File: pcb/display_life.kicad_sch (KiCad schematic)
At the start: 50 parts, among them J3 1st Bit_shifter, J4 1st 7 Segment, J5 2nd Bit_shifter, J6 2nd 7 Segment, J7 decoder_input, J8 disp_1_decoder, J9 disp_2_decoder, Q1 Q_NPN_CBE, Q2 Q_NPN_CBE, Q3 Q_NPN_CBE, Q4 Q_NPN_CBE, Q5 Q_NPN_CBE, Q6 Q_NPN_CBE, Q7 Q_NPN_CBE, Q8 Q_NPN_CBE, U2 74HC595, U3 74HC595, U4 4028, U5 CC56-12SURKWA, U6 CC56-12SURKWA

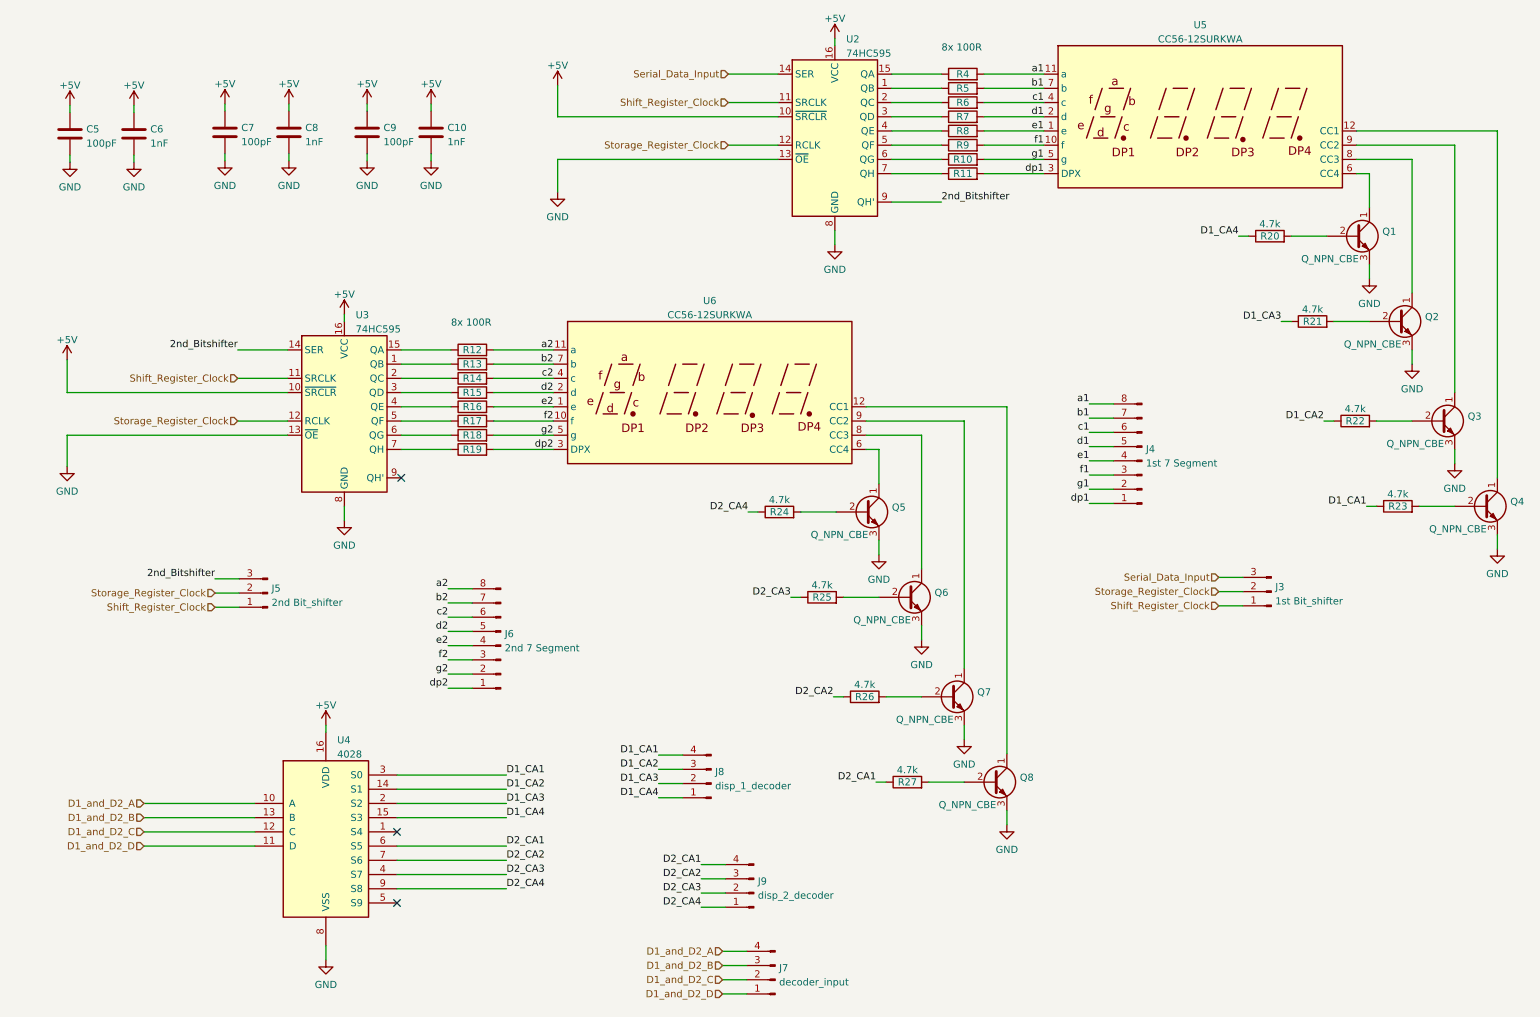
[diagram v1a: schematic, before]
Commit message: new parts and stuff
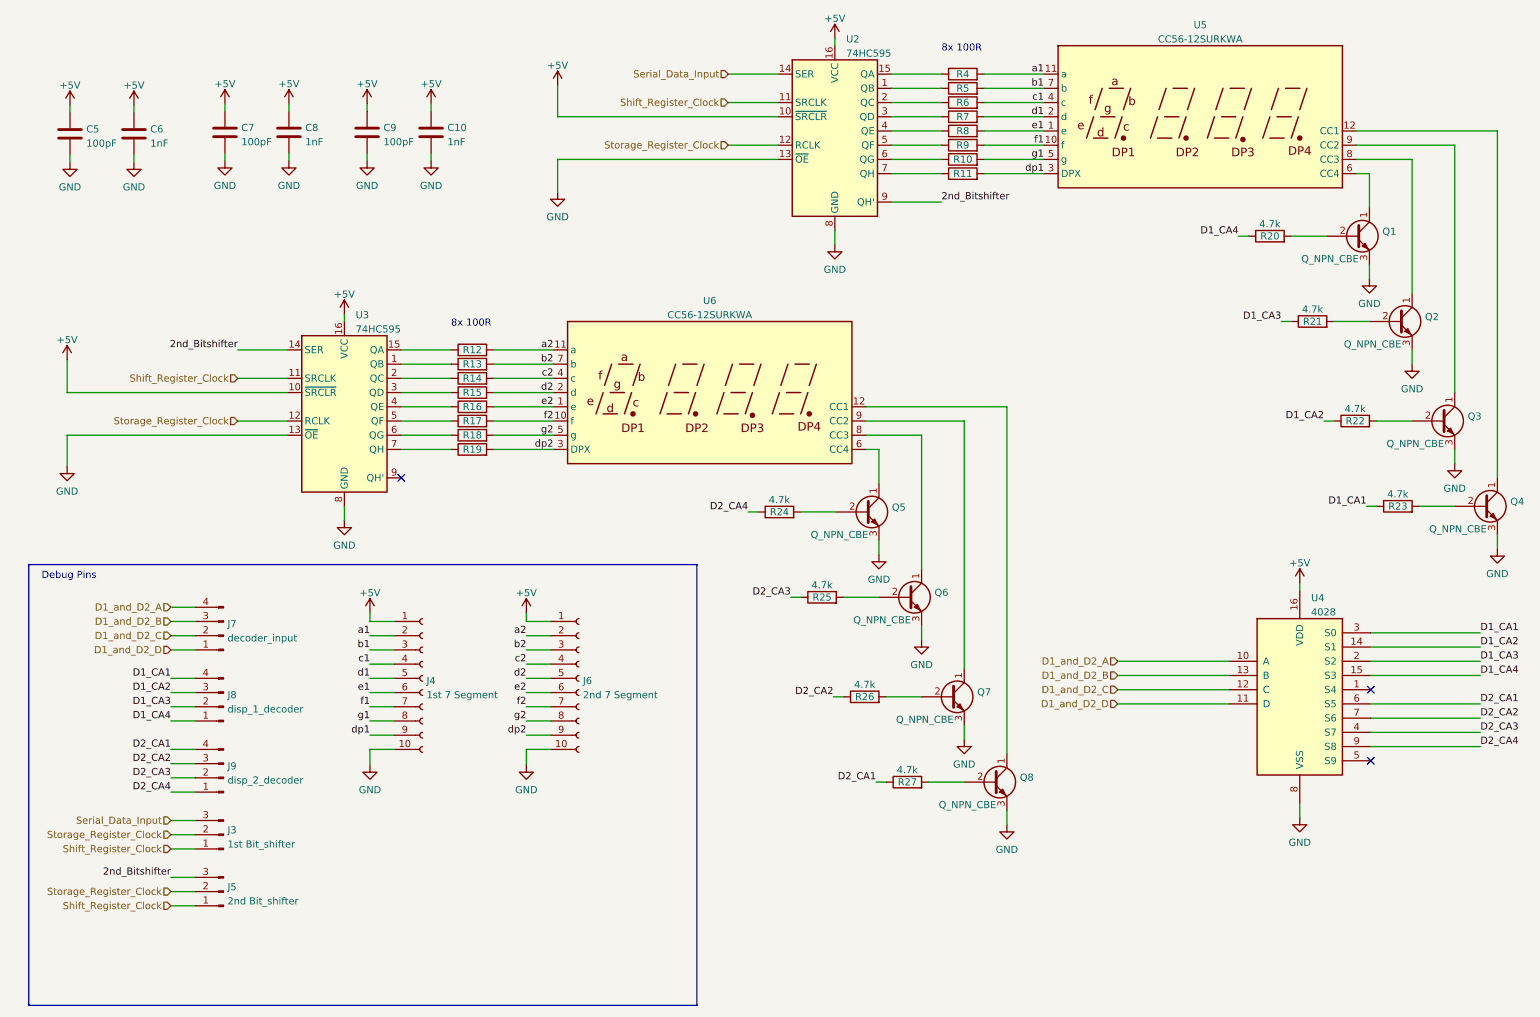
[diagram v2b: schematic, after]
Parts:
- removed J4: 1st 7 Segment, Connector_PinHeader_2.54mm:PinHeader_1x08_P2.54mm_Vertical, symbol Connector:Conn_01x08_Male
- removed J6: 2nd 7 Segment, Connector_PinHeader_2.54mm:PinHeader_1x08_P2.54mm_Vertical, symbol Connector:Conn_01x08_Male
- added J4: 1st 7 Segment, Connector_PinHeader_2.54mm:PinHeader_1x10_P2.54mm_Vertical, symbol Connector:Conn_01x10_Female
- added J6: 2nd 7 Segment, Connector_PinHeader_2.54mm:PinHeader_1x10_P2.54mm_Vertical, symbol Connector:Conn_01x10_Female
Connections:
- net +5V: now also J4.1 (Pin_1), J6.1 (Pin_1)
- net GND: now also J4.10 (Pin_10), J6.10 (Pin_10)
- net a1: now also J4.2 (Pin_2)
- net a2: now also J6.2 (Pin_2)
- net b1: now also J4.3 (Pin_3)
- net b2: now also J6.3 (Pin_3)
- net c1: now also J4.4 (Pin_4)
- net c2: now also J6.4 (Pin_4)
- net d1: now also J4.5 (Pin_5)
- net d2: now also J6.5 (Pin_5)
- net dp1: now also J4.9 (Pin_9)
- net dp2: now also J6.9 (Pin_9)
- net e1: now also J4.6 (Pin_6)
- net e2: now also J6.6 (Pin_6)
- net f1: now also J4.7 (Pin_7)
- net f2: now also J6.7 (Pin_7)
- net g1: now also J4.8 (Pin_8)
- net g2: now also J6.8 (Pin_8)
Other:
- note added: "Debug Pins"
- moved on the sheet: J3, J5, J7, J8, J9, U4

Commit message: new layout with usb
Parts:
- R10, R11, R12, R13, R14, R15, R16, R17, R18, R19, R20, R21, R22, R23, R24, R25, R26, R27, R4, R5, R6, R7, R8, R9: footprint Resistor_THT:R_Axial_DIN0207_L6.3mm_D2.5mm_P7.62mm_Horizontal -> Resistor_THT:R_Axial_DIN0207_L6.3mm_D2.5mm_P10.16mm_Horizontal
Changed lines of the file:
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@@
       (effects (font (size 1.27 1.27)) hide)
     )
-    (property "Footprint" "Resistor_THT:R_Axial_DIN0207_L6.3mm_D2.5mm_P7.62mm_Horizontal" (id 2) (at 94.488 87.884 90)
+    (property "Footprint" "Resistor_THT:R_Axial_DIN0207_L6.3mm_D2.5mm_P10.16mm_Horizontal" (id 2) (at 94.488 87.884 90)
       (effects (font (size 1.27 1.27)) hide)
     )
@@
     (property "Reference" "R21" (id 0) (at 244.602 70.866 90))
     (property "Value" "4.7k" (id 1) (at 244.602 68.6871 90))
-    (property "Footprint" "Resistor_THT:R_Axial_DIN0207_L6.3mm_D2.5mm_P7.62mm_Horizontal" (id 2) (at 244.602 72.644 90)
+    (property "Footprint" "Resistor_THT:R_Axial_DIN0207_L6.3mm_D2.5mm_P10.16mm_Horizontal" (id 2) (at 244.602 72.644 90)
       (effects (font (size 1.27 1.27)) hide)
     )
@@
     (property "Reference" "R20" (id 0) (at 236.982 55.626 90))
     (property "Value" "4.7k" (id 1) (at 236.982 53.4471 90))
-    (property "Footprint" "Resistor_THT:R_Axial_DIN0207_L6.3mm_D2.5mm_P7.62mm_Horizontal" (id 2) (at 236.982 57.404 90)
+    (property "Footprint" "Resistor_THT:R_Axial_DIN0207_L6.3mm_D2.5mm_P10.16mm_Horizontal" (id 2) (at 236.982 57.404 90)
       (effects (font (size 1.27 1.27)) hide)
     )
@@
       (effects (font (size 1.27 1.27)) hide)
     )
-    (property "Footprint" "Resistor_THT:R_Axial_DIN0207_L6.3mm_D2.5mm_P7.62mm_Horizontal" (id 2) (at 94.488 82.804 90)
+    (property "Footprint" "Resistor_THT:R_Axial_DIN0207_L6.3mm_D2.5mm_P10.16mm_Horizontal" (id 2) (at 94.488 82.804 90)
       (effects (font (size 1.27 1.27)) hide)
     )
@@
     (property "Reference" "R24" (id 0) (at 149.352 104.902 90))
     (property "Value" "4.7k" (id 1) (at 149.352 102.7231 90))
-    (property "Footprint" "Resistor_THT:R_Axial_DIN0207_L6.3mm_D2.5mm_P7.62mm_Horizontal" (id 2) (at 149.352 106.68 90)
+    (property "Footprint" "Resistor_THT:R_Axial_DIN0207_L6.3mm_D2.5mm_P10.16mm_Horizontal" (id 2) (at 149.352 106.68 90)
       (effects (font (size 1.27 1.27)) hide)
     )
@@
       (effects (font (size 1.27 1.27)) hide)
     )
-    (property "Footprint" "Resistor_THT:R_Axial_DIN0207_L6.3mm_D2.5mm_P7.62mm_Horizontal" (id 2) (at 182.118 30.988 90)
+    (property "Footprint" "Resistor_THT:R_Axial_DIN0207_L6.3mm_D2.5mm_P10.16mm_Horizontal" (id 2) (at 182.118 30.988 90)
       (effects (font (size 1.27 1.27)) hide)
     )
@@
     (property "Reference" "R23" (id 0) (at 259.842 103.886 90))
     (property "Value" "4.7k" (id 1) (at 259.842 101.7071 90))
-    (property "Footprint" "Resistor_THT:R_Axial_DIN0207_L6.3mm_D2.5mm_P7.62mm_Horizontal" (id 2) (at 259.842 105.664 90)
+    (property "Footprint" "Resistor_THT:R_Axial_DIN0207_L6.3mm_D2.5mm_P10.16mm_Horizontal" (id 2) (at 259.842 105.664 90)
       (effects (font (size 1.27 1.27)) hide)
     )
@@
     (property "Reference" "R25" (id 0) (at 156.972 120.142 90))
     (property "Value" "4.7k" (id 1) (at 156.972 117.9631 90))
-    (property "Footprint" "Resistor_THT:R_Axial_DIN0207_L6.3mm_D2.5mm_P7.62mm_Horizontal" (id 2) (at 156.972 121.92 90)
+    (property "Footprint" "Resistor_THT:R_Axial_DIN0207_L6.3mm_D2.5mm_P10.16mm_Horizontal" (id 2) (at 156.972 121.92 90)
       (effects (font (size 1.27 1.27)) hide)
     )
@@
       (effects (font (size 1.27 1.27)) hide)
     )
-    (property "Footprint" "Resistor_THT:R_Axial_DIN0207_L6.3mm_D2.5mm_P7.62mm_Horizontal" (id 2) (at 182.118 46.228 90)
+    (property "Footprint" "Resistor_THT:R_Axial_DIN0207_L6.3mm_D2.5mm_P10.16mm_Horizontal" (id 2) (at 182.118 46.228 90)
       (effects (font (size 1.27 1.27)) hide)
     )
@@
     (property "Reference" "R26" (id 0) (at 164.592 137.922 90))
     (property "Value" "4.7k" (id 1) (at 164.592 135.7431 90))
-    (property "Footprint" "Resistor_THT:R_Axial_DIN0207_L6.3mm_D2.5mm_P7.62mm_Horizontal" (id 2) (at 164.592 139.7 90)
+    (property "Footprint" "Resistor_THT:R_Axial_DIN0207_L6.3mm_D2.5mm_P10.16mm_Horizontal" (id 2) (at 164.592 139.7 90)
       (effects (font (size 1.27 1.27)) hide)
     )
@@
       (effects (font (size 1.27 1.27)) hide)
     )
-    (property "Footprint" "Resistor_THT:R_Axial_DIN0207_L6.3mm_D2.5mm_P7.62mm_Horizontal" (id 2) (at 182.118 36.068 90)
+    (property "Footprint" "Resistor_THT:R_Axial_DIN0207_L6.3mm_D2.5mm_P10.16mm_Horizontal" (id 2) (at 182.118 36.068 90)
       (effects (font (size 1.27 1.27)) hide)
     )
@@
       (effects (font (size 1.27 1.27)) hide)
     )
-    (property "Footprint" "Resistor_THT:R_Axial_DIN0207_L6.3mm_D2.5mm_P7.62mm_Horizontal" (id 2) (at 94.488 77.724 90)
+    (property "Footprint" "Resistor_THT:R_Axial_DIN0207_L6.3mm_D2.5mm_P10.16mm_Horizontal" (id 2) (at 94.488 77.724 90)
       (effects (font (size 1.27 1.27)) hide)
     )
@@
       (effects (font (size 1.27 1.27)) hide)
     )
-    (property "Footprint" "Resistor_THT:R_Axial_DIN0207_L6.3mm_D2.5mm_P7.62mm_Horizontal" (id 2) (at 94.488 80.264 90)
+    (property "Footprint" "Resistor_THT:R_Axial_DIN0207_L6.3mm_D2.5mm_P10.16mm_Horizontal" (id 2) (at 94.488 80.264 90)
       (effects (font (size 1.27 1.27)) hide)
     )
@@
       (effects (font (size 1.27 1.27)) hide)
     )
-    (property "Footprint" "Resistor_THT:R_Axial_DIN0207_L6.3mm_D2.5mm_P7.62mm_Horizontal" (id 2) (at 94.488 90.424 90)
+    (property "Footprint" "Resistor_THT:R_Axial_DIN0207_L6.3mm_D2.5mm_P10.16mm_Horizontal" (id 2) (at 94.488 90.424 90)
       (effects (font (size 1.27 1.27)) hide)
     )
@@
       (effects (font (size 1.27 1.27)) hide)
     )
-    (property "Footprint" "Resistor_THT:R_Axial_DIN0207_L6.3mm_D2.5mm_P7.62mm_Horizontal" (id 2) (at 94.488 85.344 90)
+    (property "Footprint" "Resistor_THT:R_Axial_DIN0207_L6.3mm_D2.5mm_P10.16mm_Horizontal" (id 2) (at 94.488 85.344 90)
       (effects (font (size 1.27 1.27)) hide)
     )
@@
       (effects (font (size 1.27 1.27)) hide)
     )
-    (property "Footprint" "Resistor_THT:R_Axial_DIN0207_L6.3mm_D2.5mm_P7.62mm_Horizontal" (id 2) (at 182.118 41.148 90)
+    (property "Footprint" "Resistor_THT:R_Axial_DIN0207_L6.3mm_D2.5mm_P10.16mm_Horizontal" (id 2) (at 182.118 41.148 90)
       (effects (font (size 1.27 1.27)) hide)
     )
@@
       (effects (font (size 1.27 1.27)) hide)
     )
-    (property "Footprint" "Resistor_THT:R_Axial_DIN0207_L6.3mm_D2.5mm_P7.62mm_Horizontal" (id 2) (at 94.488 92.964 90)
+    (property "Footprint" "Resistor_THT:R_Axial_DIN0207_L6.3mm_D2.5mm_P10.16mm_Horizontal" (id 2) (at 94.488 92.964 90)
       (effects (font (size 1.27 1.27)) hide)
     )
@@
       (effects (font (size 1.27 1.27)) hide)
     )
-    (property "Footprint" "Resistor_THT:R_Axial_DIN0207_L6.3mm_D2.5mm_P7.62mm_Horizontal" (id 2) (at 182.118 28.448 90)
+    (property "Footprint" "Resistor_THT:R_Axial_DIN0207_L6.3mm_D2.5mm_P10.16mm_Horizontal" (id 2) (at 182.118 28.448 90)
       (effects (font (size 1.27 1.27)) hide)
     )
@@
       (effects (font (size 1.27 1.27)) hide)
     )
-    (property "Footprint" "Resistor_THT:R_Axial_DIN0207_L6.3mm_D2.5mm_P7.62mm_Horizontal" (id 2) (at 182.118 38.608 90)
+    (property "Footprint" "Resistor_THT:R_Axial_DIN0207_L6.3mm_D2.5mm_P10.16mm_Horizontal" (id 2) (at 182.118 38.608 90)
       (effects (font (size 1.27 1.27)) hide)
     )
@@
       (effects (font (size 1.27 1.27)) hide)
     )
-    (property "Footprint" "Resistor_THT:R_Axial_DIN0207_L6.3mm_D2.5mm_P7.62mm_Horizontal" (id 2) (at 182.118 43.688 90)
+    (property "Footprint" "Resistor_THT:R_Axial_DIN0207_L6.3mm_D2.5mm_P10.16mm_Horizontal" (id 2) (at 182.118 43.688 90)
       (effects (font (size 1.27 1.27)) hide)
     )
@@
       (effects (font (size 1.27 1.27)) hide)
     )
-    (property "Footprint" "Resistor_THT:R_Axial_DIN0207_L6.3mm_D2.5mm_P7.62mm_Horizontal" (id 2) (at 182.118 33.528 90)
+    (property "Footprint" "Resistor_THT:R_Axial_DIN0207_L6.3mm_D2.5mm_P10.16mm_Horizontal" (id 2) (at 182.118 33.528 90)
       (effects (font (size 1.27 1.27)) hide)
     )
@@
     (property "Reference" "R27" (id 0) (at 172.212 153.162 90))
     (property "Value" "4.7k" (id 1) (at 172.212 150.9831 90))
-    (property "Footprint" "Resistor_THT:R_Axial_DIN0207_L6.3mm_D2.5mm_P7.62mm_Horizontal" (id 2) (at 172.212 154.94 90)
+    (property "Footprint" "Resistor_THT:R_Axial_DIN0207_L6.3mm_D2.5mm_P10.16mm_Horizontal" (id 2) (at 172.212 154.94 90)
       (effects (font (size 1.27 1.27)) hide)
     )
@@
       (effects (font (size 1.27 1.27)) hide)
     )
-    (property "Footprint" "Resistor_THT:R_Axial_DIN0207_L6.3mm_D2.5mm_P7.62mm_Horizontal" (id 2) (at 94.488 95.504 90)
+    (property "Footprint" "Resistor_THT:R_Axial_DIN0207_L6.3mm_D2.5mm_P10.16mm_Horizontal" (id 2) (at 94.488 95.504 90)
       (effects (font (size 1.27 1.27)) hide)
     )
@@
     (property "Reference" "R22" (id 0) (at 252.222 88.646 90))
     (property "Value" "4.7k" (id 1) (at 252.222 86.4671 90))
-    (property "Footprint" "Resistor_THT:R_Axial_DIN0207_L6.3mm_D2.5mm_P7.62mm_Horizontal" (id 2) (at 252.222 90.424 90)
-      (effects (font (size 1.27 1.27)) hide)
-    )
+    (property "Footprint" "Resistor_THT:R_Axial_DIN0207_L6.3mm_D2.5mm_P10.16mm_Horizontal" (id 2) (at 252.222 90.424 90)
+      (effects (font (size 1.27 1.27)) hide)
+    )
